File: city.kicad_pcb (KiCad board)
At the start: 2 copper layers, 34 x 38 mm, 29 parts, among them J1 USB_C_Receptacle_USB2.0_16P, J4 Conn_01x08_Pin, J5 Conn_01x08_Pin, SW1 SW_Push, SW2 SW_Push, U1 USBLC6-2SC6, U2 AP2112K-3.3, U3 ESP32-C3-WROOM-02, Y1 Crystal

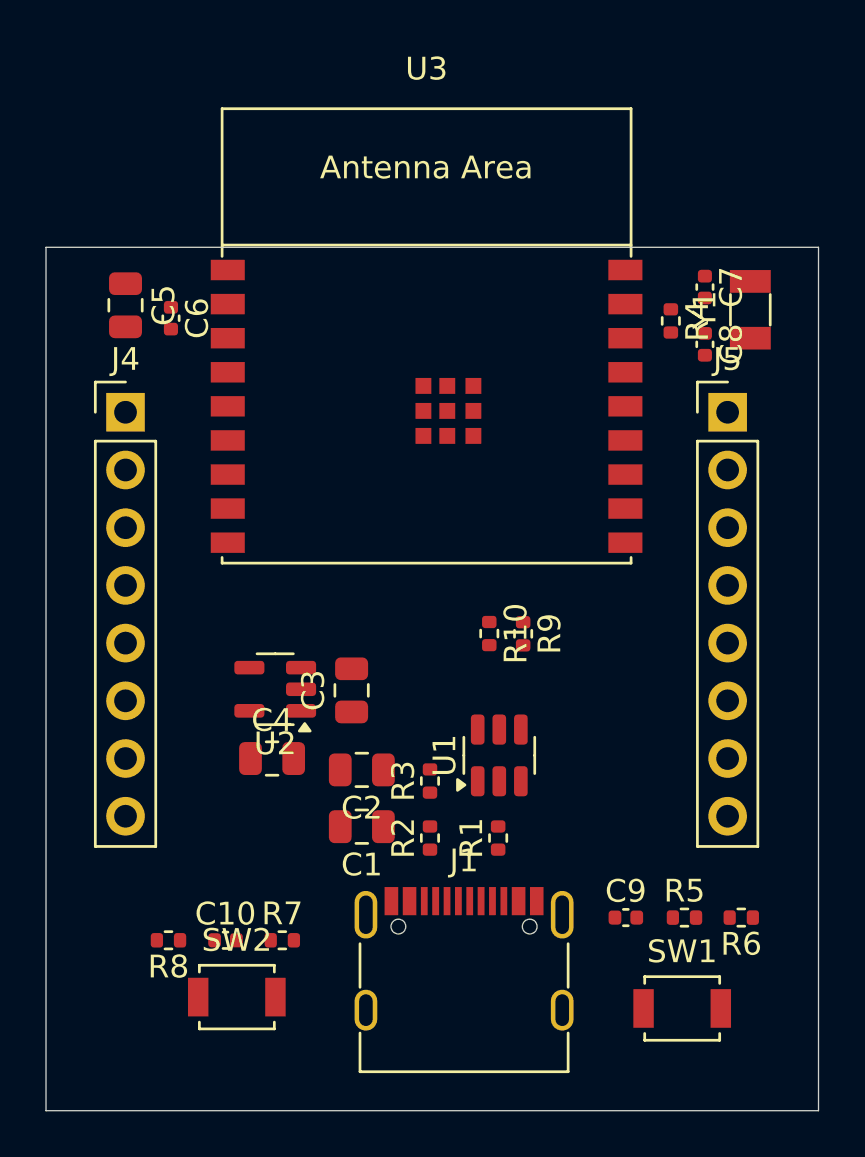
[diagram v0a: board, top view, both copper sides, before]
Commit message: after routing
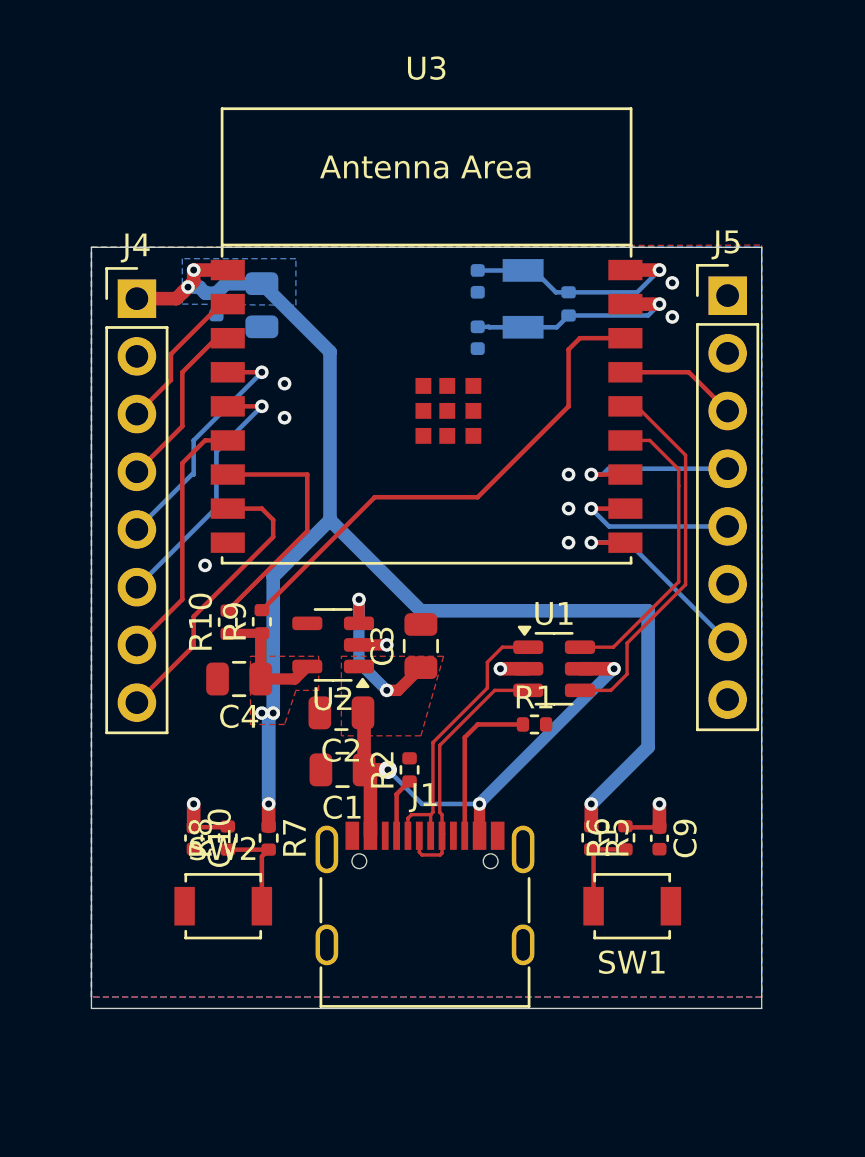
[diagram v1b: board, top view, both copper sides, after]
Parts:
- removed R3: 0R, Resistor_SMD:R_0402_1005Metric
- C5, C6, C7, C8, R4, Y1: moved to B.Cu
- moved R10 11.5 mm to (37.5, 75.0), turned to 90 degrees
- moved R9 11.5 mm to (39.0, 75.0), turned to 90 degrees
- moved Y1 10.0 mm to (50.5, 60.8)
- moved C8 10.0 mm to (48.5, 62.5)
- moved C7 10.0 mm to (48.5, 60.0)
- moved R6 6.19 mm to (55.0, 84.5), turned to 90 degrees
- moved C5 6.00 mm to (39.0, 61.0)
- moved R5 5.40 mm to (53.5, 84.5), turned to -90 degrees
- moved R1 5.25 mm to (51.0, 79.5), turned to 0 degrees
- moved R8 5.20 mm to (37.5, 84.5), turned to 90 degrees
- moved J5 5.14 mm to (59.5, 60.6)
- moved J4 5.02 mm to (33.5, 60.8)
- moved SW1 5.01 mm to (55.3, 87.5), turned to 180 degrees
- moved C10 4.71 mm to (36.0, 84.5), turned to -90 degrees
- moved R4 4.56 mm to (52.5, 61.0)
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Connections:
- C1 pad 1: VBUS -> +5V
- J1 pad A4: VBUS -> +5V
- J1 pad A9: VBUS -> +5V
- J1 pad B4: VBUS -> +5V
- J1 pad B9: VBUS -> +5V
- U1 pad 5: VBUS -> +5V
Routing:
- net +3.3V: track 0.00 -> 67.3 mm, vias 0 -> 6
- net +5V: track 0.00 -> 48.5 mm, vias 0 -> 5
- net EN: track 0.00 -> 39.3 mm, vias 0 -> 1
- net IO2: track 0.00 -> 22.4 mm
- net IO9: track 0.00 -> 20.7 mm, vias 0 -> 1
- net USB_D+: track 0.00 -> 16.9 mm
- net USB_D-: track 0.00 -> 13.7 mm
- net /D-: track 0.00 -> 12.7 mm
- net IO6: track 0.00 -> 12.0 mm, vias 0 -> 1
- net /D+: track 0.00 -> 11.6 mm
- net IO8: track 0.00 -> 11.4 mm
- net IO7: track 0.00 -> 11.2 mm
- net IO5: track 0.00 -> 10.7 mm, vias 0 -> 1
- net Net-(U3-GPIO0/ADC1_CH0/XTAL_32K_P): track 0.00 -> 10.3 mm, vias 0 -> 1
- net Net-(U3-GPIO1/ADC1_CH1/XTAL_32K_N): track 0.00 -> 9.93 mm, vias 0 -> 1
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- added copper zone on B.Cu, net +3.3V
- added copper zone on F.Cu, net +3.3V
- added copper zone on F.Cu, net +5V
- added copper zone on B.Cu, net GND
- added copper zone on F.Cu, net GND
- added copper zone on In1.Cu, net GND
- added copper zone on In2.Cu, net GND
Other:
- board size 34 x 38 mm -> 29.5 x 33.5 mm
- copper layers 2 -> 4
